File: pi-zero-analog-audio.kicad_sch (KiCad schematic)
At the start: 6 parts, among them J1 GPIO, U1 CAT24C256

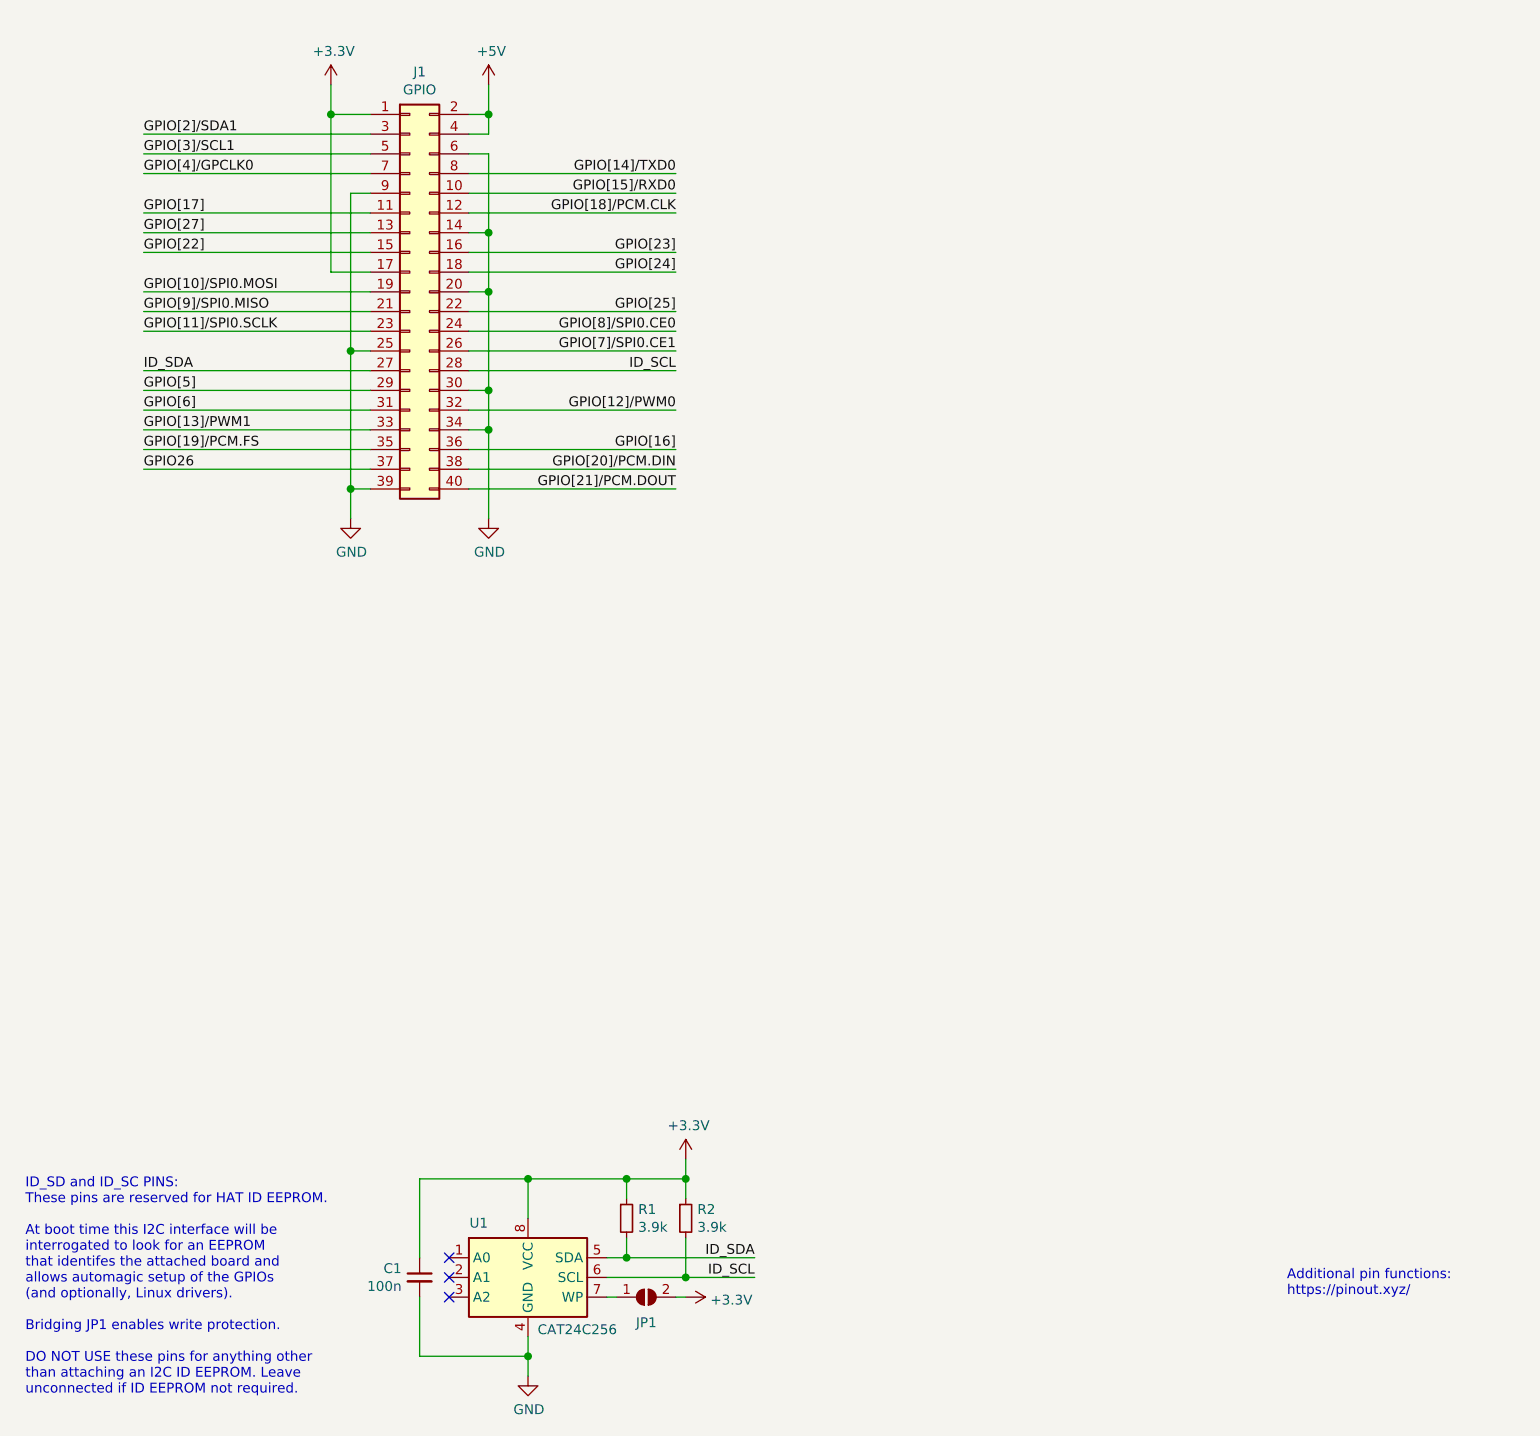
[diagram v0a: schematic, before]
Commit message: Unrouted
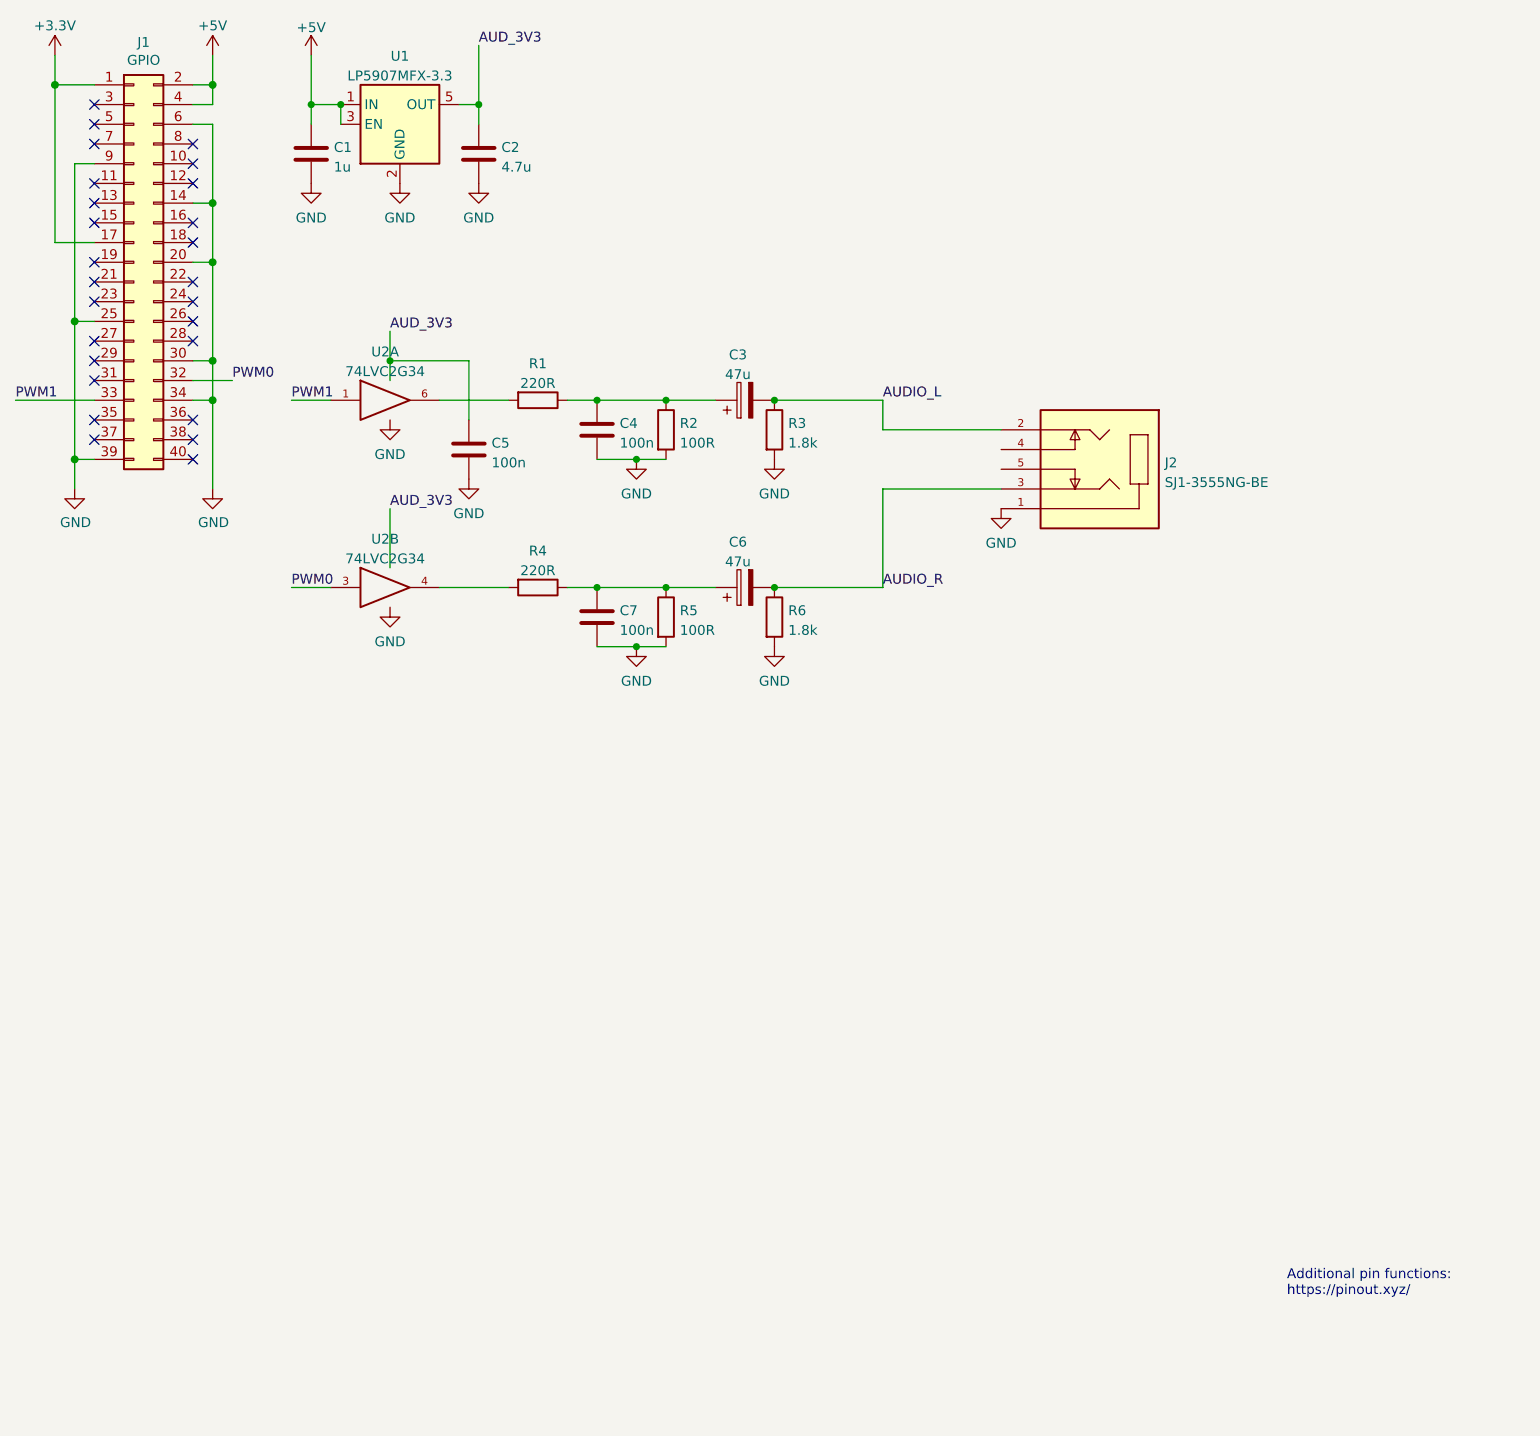
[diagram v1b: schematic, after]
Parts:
- removed C1: 100n, symbol Device:C_Small
- removed JP1: ID_WP, symbol Jumper:SolderJumper_2_Open
- removed R1, R2: 3.9k, symbol Device:R_Small
- removed U1: CAT24C256, symbol Memory_EEPROM:CAT24C256
- added C1: 1u, Capacitor_SMD:C_0805_2012Metric_Pad1.18x1.45mm_HandSolder, symbol Device:C
- added C2: 4.7u, Capacitor_SMD:C_0805_2012Metric_Pad1.18x1.45mm_HandSolder, symbol Device:C
- added C3, C6: 47u, Capacitor_SMD:C_0805_2012Metric_Pad1.18x1.45mm_HandSolder, symbol Device:C_Polarized
- added C4, C5, C7: 100n, Capacitor_SMD:C_0805_2012Metric_Pad1.18x1.45mm_HandSolder, symbol Device:C
- added J2: SJ1-3555NG-BE, CUI_SJ1-3555NG-BE, symbol SJ1-3555NG-BE:SJ1-3555NG-BE
- added R1, R4: 220R, Resistor_SMD:R_0805_2012Metric_Pad1.20x1.40mm_HandSolder, symbol Device:R
- added R2, R5: 100R, Resistor_SMD:R_0805_2012Metric_Pad1.20x1.40mm_HandSolder, symbol Device:R
- added R3, R6: 1.8k, Resistor_SMD:R_0805_2012Metric_Pad1.20x1.40mm_HandSolder, symbol Device:R
- added U1: LP5907MFX-3.3, Package_TO_SOT_SMD:SOT-23-5, symbol Regulator_Linear:LP5907MFX-3.3
- added U2: 74LVC2G34, Package_TO_SOT_SMD:SOT-23-6_Handsoldering, symbol 74xGxx:74LVC2G34
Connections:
- net +5V: now also C1.1, U1.1 (IN), U1.3 (EN)
- net GND: now also C1.2, C2.2, C4.2, C5.2, C7.2, J2.1, R2.2, R3.2, R5.2, R6.2, U1.2 (GND), U2.2 (GND), U2.2 (GND)
- net +3V3 renamed +3.3V
- net GPIO26: no longer names the net of J1.37 (Pin_37)
- net GPIO[10]/SPI0.MOSI: no longer names the net of J1.19 (Pin_19)
- net GPIO[11]/SPI0.SCLK: no longer names the net of J1.23 (Pin_23)
- net GPIO[12]/PWM0 renamed PWM0
- net PWM0: now also U2.3
- net GPIO[13]/PWM1 renamed PWM1
- net PWM1: now also U2.1
- net GPIO[14]/TXD0: no longer names the net of J1.8 (Pin_8)
- net GPIO[15]/RXD0: no longer names the net of J1.10 (Pin_10)
- net GPIO[16]: no longer names the net of J1.36 (Pin_36)
- net GPIO[17]: no longer names the net of J1.11 (Pin_11)
- net GPIO[18]/PCM.CLK: no longer names the net of J1.12 (Pin_12)
- net GPIO[19]/PCM.FS: no longer names the net of J1.35 (Pin_35)
- net GPIO[20]/PCM.DIN: no longer names the net of J1.38 (Pin_38)
- net GPIO[21]/PCM.DOUT: no longer names the net of J1.40 (Pin_40)
- net GPIO[22]: no longer names the net of J1.15 (Pin_15)
- net GPIO[23]: no longer names the net of J1.16 (Pin_16)
- net GPIO[24]: no longer names the net of J1.18 (Pin_18)
- net GPIO[25]: no longer names the net of J1.22 (Pin_22)
- net GPIO[27]: no longer names the net of J1.13 (Pin_13)
- net GPIO[2]/SDA1: no longer names the net of J1.3 (Pin_3)
- net GPIO[3]/SCL1: no longer names the net of J1.5 (Pin_5)
- net GPIO[4]/GPCLK0: no longer names the net of J1.7 (Pin_7)
- net GPIO[5]: no longer names the net of J1.29 (Pin_29)
- net GPIO[6]: no longer names the net of J1.31 (Pin_31)
- net GPIO[7]/SPI0.CE1: no longer names the net of J1.26 (Pin_26)
- net GPIO[8]/SPI0.CE0: no longer names the net of J1.24 (Pin_24)
- net GPIO[9]/SPI0.MISO: no longer names the net of J1.21 (Pin_21)
- net ID_SCL: no longer names the net of J1.28 (Pin_28)
- net ID_SDA: no longer names the net of J1.27 (Pin_27)
- new net: R1.2, U2.6
- new net: C6.1, C7.1, R4.1, R5.1
- new net: R4.2, U2.4
- new net: C3.1, C4.1, R1.1, R2.1
- new net AUDIO_L: C3.2, J2.2, R3.1
- new net AUDIO_R: C6.2, J2.3, R6.1
- new net VCC: C2.1, C5.1, U1.5 (OUT), U2.5 (VCC), U2.5 (VCC)
- no-connect marks 3 -> 26
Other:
- note removed: "ID_SD and ID_SC PINS: These pins are reserved for HAT ID EEPROM. At boot time this I2C interface will be interrogated to look for an EEPROM that identifes the attached board and allows automagic setup of the GPIOs (and optionally, Linux drivers). Bridging JP1 enables write protection. DO NOT USE these pins for anything other than attaching an I2C ID EEPROM. Leave unconnected if ID EEPROM not requ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"
- moved on the sheet: J1
